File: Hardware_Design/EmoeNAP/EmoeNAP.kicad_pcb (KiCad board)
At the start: 4 copper layers, 75 x 36 mm, 149 parts, among them J1 Power, J2 10Hz to WIDEBAND, J3 10Hz to 1MHz, J4 Input, J5 10Hz to 100kHz, U1 OPA1612, U2 OPA1612, U3 OPA1612, U4 PS-12E05, U5 OPA1612, U6 OPA1679, U7 OPA1612, U8 OPA1612

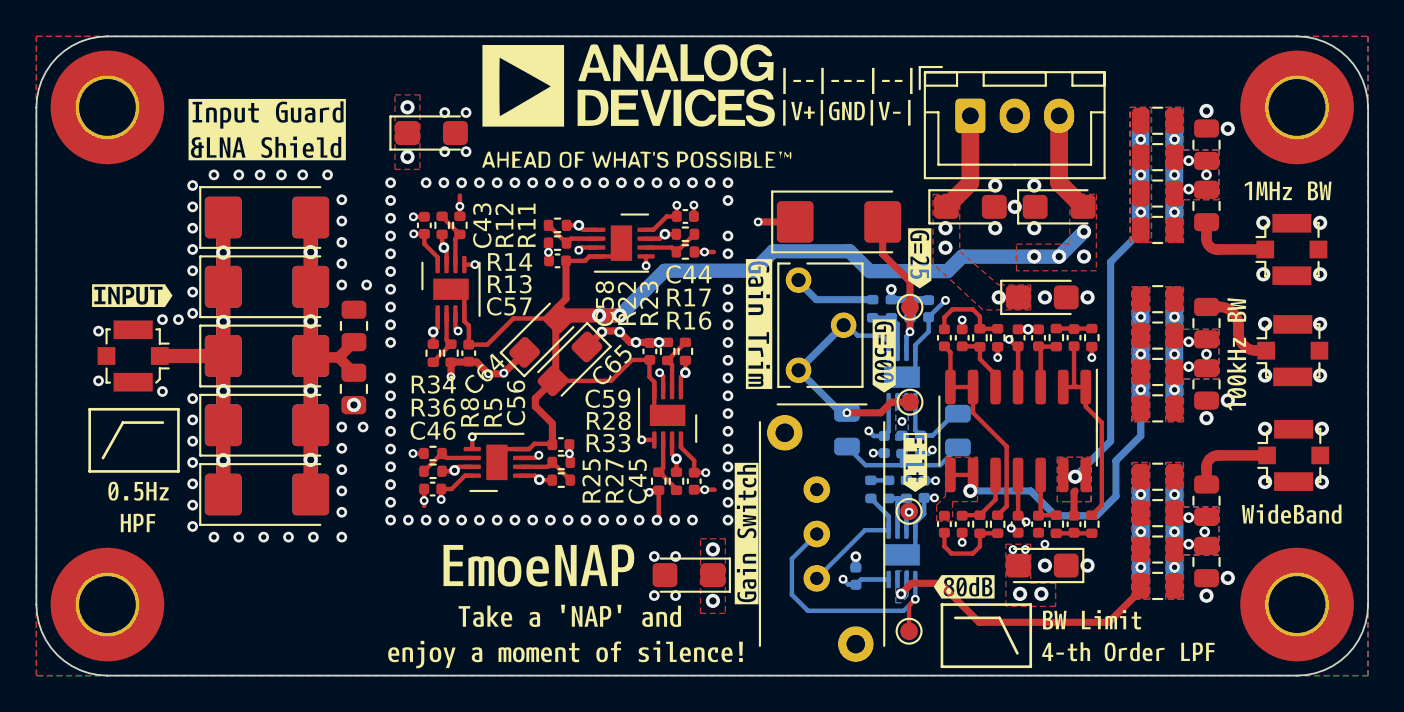
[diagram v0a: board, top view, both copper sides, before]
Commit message: Update EmoeNAP design
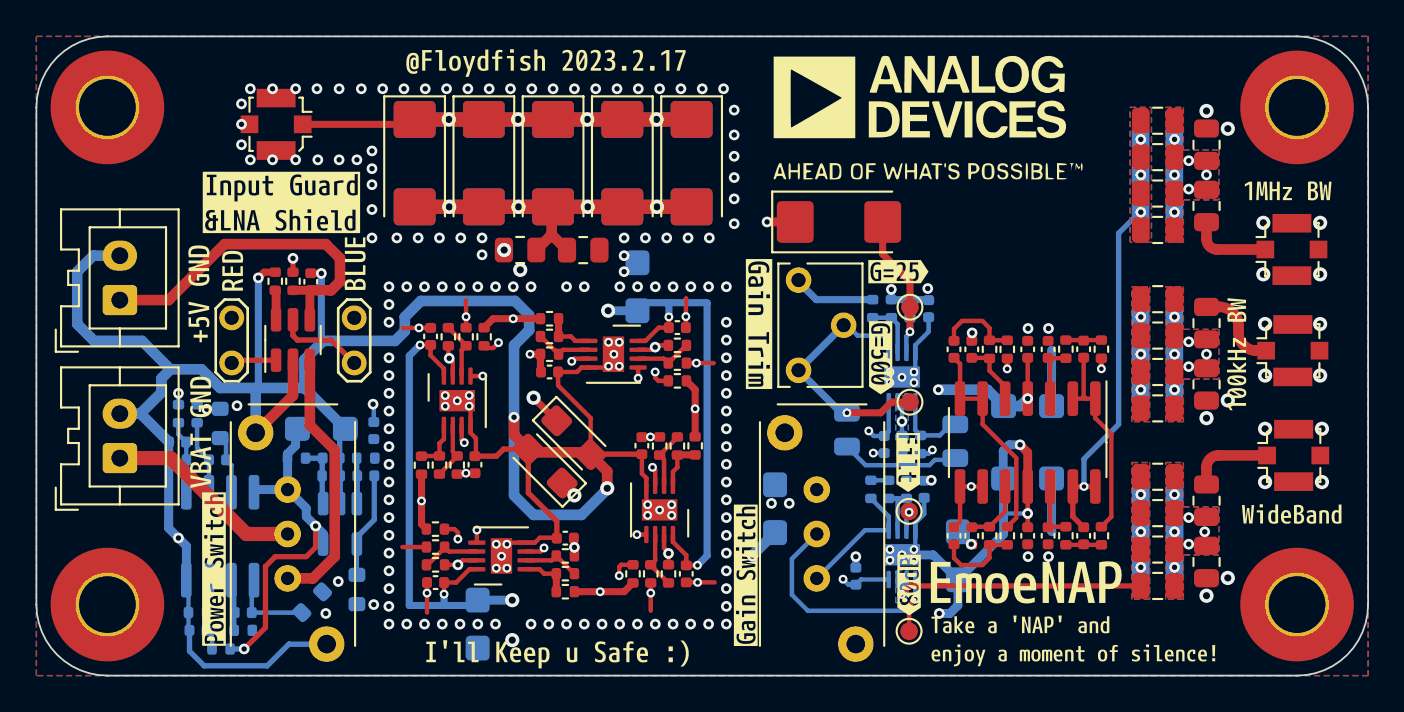
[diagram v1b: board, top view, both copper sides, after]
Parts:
- removed kibuzzard-6378A5E8: G***, kibuzzard-6378A5E8
- removed kibuzzard-6378A61B: G***, kibuzzard-6378A61B
- removed kibuzzard-6378A7B0: G***, kibuzzard-6378A7B0
- removed kibuzzard-6378A846: G***, kibuzzard-6378A846
- removed kibuzzard-6378A8BF: G***, kibuzzard-6378A8BF
- removed kibuzzard-6378AB08: G***, kibuzzard-6378AB08
- added C65: 2.2uF, Capacitor_Tantalum_SMD:CP_EIA-3216-10_Kemet-I, B.Cu at (126.0, 111.1)
- added C66: 100pF, Capacitor_SMD:C_0402_1005Metric, B.Cu at (119.1, 122.5)
- added C67: 100pF, Capacitor_SMD:C_0402_1005Metric, B.Cu at (121.7, 121.5)
- added C68: 100pF, Capacitor_SMD:C_0402_1005Metric, B.Cu at (118.0, 111.8)
- added C69: 100pF, Capacitor_SMD:C_0402_1005Metric, B.Cu at (120.2, 112.8)
- added C70: 0.1uF, Capacitor_SMD:C_0402_1005Metric, B.Cu at (129.0, 111.2)
- added C71: 0.1uF, Capacitor_SMD:C_0402_1005Metric, F.Cu at (125.5, 102.8)
- added C72: 100pF, Capacitor_SMD:C_0402_1005Metric, B.Cu at (126.6, 112.8)
- added C73: 100pF, Capacitor_SMD:C_0402_1005Metric, B.Cu at (128.6, 113.8)
- added J6: GREEN, TestPoint:TestPoint_2Pads_Pitch2.54mm_Drill0.8mm, F.Cu at (127.9, 104.9)
- added J7: RED, TestPoint:TestPoint_2Pads_Pitch2.54mm_Drill0.8mm, F.Cu at (121.0, 104.8)
- added J8: USB_CHR, Connector_JST:JST_XA_B02B-XASK-1_1x02_P2.50mm_Vertical, F.Cu at (114.7, 103.8)
- added R12: 1R, Resistor_SMD:R_0402_1005Metric, F.Cu at (146.1, 108.4)
- added R15: 1R, Resistor_SMD:R_0402_1005Metric, F.Cu at (147.1, 112.1)
- added R18: 1R, Resistor_SMD:R_0402_1005Metric, F.Cu at (143.6, 119.3)
- added R24: 1R, Resistor_SMD:R_0402_1005Metric, F.Cu at (139.8, 120.3)
- added R3: 1R, Resistor_SMD:R_0402_1005Metric, F.Cu at (138.9, 104.9)
- added R30: 1R, Resistor_SMD:R_0402_1005Metric, F.Cu at (132.5, 116.7)
- added R34: 1R, Resistor_SMD:R_0402_1005Metric, F.Cu at (131.7, 113.1)
- added R41: 1R, Resistor_SMD:R_0402_1005Metric, F.Cu at (135.2, 105.9)
- added R45: 10k, Resistor_SMD:R_0402_1005Metric, B.Cu at (120.4, 123.5)
- added R46: 10k, Resistor_SMD:R_0402_1005Metric, B.Cu at (119.1, 121.5)
- added R47: 1k, Resistor_SMD:R_0402_1005Metric, B.Cu at (121.7, 122.5)
- added R48: 10k, Resistor_SMD:R_0402_1005Metric, B.Cu at (118.0, 110.2)
- added R49: 10k, Resistor_SMD:R_0402_1005Metric, B.Cu at (117.9, 112.8)
- added R50: 1k, Resistor_SMD:R_0402_1005Metric, B.Cu at (119.0, 110.2)
- added R51: 2k, Resistor_SMD:R_0402_1005Metric, F.Cu at (123.5, 102.8)
- added R52: 1k, Resistor_SMD:R_0402_1005Metric, F.Cu at (124.5, 102.8)
- added R53: 10k, Resistor_SMD:R_0402_1005Metric, B.Cu at (124.7, 112.8)
- added R54: 10k, Resistor_SMD:R_0402_1005Metric, B.Cu at (126.6, 113.8)
- added R55: 1k, Resistor_SMD:R_0402_1005Metric, B.Cu at (128.6, 112.8)
- added RISO5: 100R, Resistor_SMD:R_0603_1608Metric, B.Cu at (125.5, 120.9)
- added RISO6: 100R, Resistor_SMD:R_0603_1608Metric, B.Cu at (120.3, 110.8)
- added RISO7: 100R, Resistor_SMD:R_0603_1608Metric, B.Cu at (128.1, 120.2)
- added U10: PS-12E05, EmoeNAP_FootPrint_Lib:PS-12E05, F.Cu at (124.2, 114.5)
- added U11: TP4057, Package_TO_SOT_SMD:SOT-23-6, F.Cu at (124.5, 106.1)
- added U12: SGM321, Package_TO_SOT_SMD:SOT-23-5, B.Cu at (127.1, 116.5)
- added U9: LT1364, Package_SO:SOIC-8_3.9x4.9mm_P1.27mm, B.Cu at (120.3, 117.2)
- added kibuzzard-63ED0A5F: G***, kibuzzard-63ED0A5F, F.Cu at (168.4, 123.0)
- added kibuzzard-63EE512D: G***, kibuzzard-63EE512D, F.Cu at (120.0, 119.0)
- added kibuzzard-63EE51C1: G***, kibuzzard-63EE51C1, F.Cu at (119.2, 103.5)
- added kibuzzard-63EE51DC: G***, kibuzzard-63EE51DC, F.Cu at (119.2, 111.3)
- added kibuzzard-63EE520C: G***, kibuzzard-63EE520C, F.Cu at (121.0, 102.2)
- added kibuzzard-63EE5216: G***, kibuzzard-63EE5216, F.Cu at (128.0, 101.8)
- added kibuzzard-63EE5345: G***, kibuzzard-63EE5345, F.Cu at (138.7, 90.5)
- added kibuzzard-63EE53DB: G***, kibuzzard-63EE53DB, F.Cu at (139.3, 123.8)
- C50: renamed from C51; moved to B.Cu
- C51: renamed from C52; moved to B.Cu
- C52: renamed from C53; moved to B.Cu
- C53: renamed from C54; moved to B.Cu
- C63: renamed from C66; moved to B.Cu
- C64: renamed from C67; moved to B.Cu
- G***: moved to B.Cu
- J1: value Power -> Battery; footprint Connector_JST:JST_XH_B3B-XH-A_1x03_P2.50mm_Vertical -> Connector_JST:JST_XA_B02B-XASK-1_1x02_P2.50mm_Vertical
- moved J1 51.6 mm to (114.7, 112.8), turned to 90 degrees
- moved G*** 51.3 mm to (165.6, 101.0)
- moved G*** 36.5 mm to (155.2, 95.8), turned to 180 degrees
- moved kibuzzard-6378A590 27.5 mm to (165.8, 119.8)
- moved C20 24.1 mm to (146.9, 96.1), turned to -90 degrees
- moved C23 24.1 mm to (146.9, 96.1), turned to -90 degrees
- moved C18 21.2 mm to (143.0, 96.1), turned to -90 degrees
- moved C26 21.2 mm to (143.0, 96.1), turned to -90 degrees
- moved C64 20.5 mm to (161.9, 118.2), turned to -90 degrees
- moved C11 20.4 mm to (131.3, 96.1), turned to -90 degrees
- moved C31 20.4 mm to (131.3, 96.1), turned to -90 degrees
- moved C53 20.2 mm to (151.6, 115.6), turned to 90 degrees
- moved C44 20.1 mm to (146.6, 119.3), turned to -90 degrees
- moved C15 19.4 mm to (139.1, 96.1), turned to -90 degrees
- moved C28 19.4 mm to (139.1, 96.1), turned to -90 degrees
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- renumbered C56 to C54, C57 to C55, C58 to C56, C59 to C57, C60 to C58, C61 to C59, C62 to C60, C64 to C61, C65 to C62, R9 to R10, R10 to R11, R11 to R13, R12 to R14, R13 to R16, R14 to R17, R15 to R19, R16 to R20, R17 to R21, R18 to R22, R19 to R23, R20 to R25, R21 to R26, R22 to R27, R23 to R28, R24 to R29, R25 to R31, R26 to R32, R27 to R33, R28 to R35, R29 to R36, R30 to R37, R31 to R38, R32 to R39, R3 to R4, R33 to R40, R34 to R42, R35 to R43, R36 to R44, R4 to R5, R5 to R6, R6 to R7, R7 to R8, R8 to R9, TP4 to TP3, TP3 to TP4
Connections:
- J1 pad 1: VDD -> /VBAT
- J1 pad 2: GND -> VSS
- R14 pad 1: Net-(C1-Pad1) -> Net-(R12-Pad1)
- R17 pad 1: Net-(C1-Pad1) -> Net-(R15-Pad1)
- R21 pad 1: Net-(C1-Pad1) -> Net-(R18-Pad1)
- R28 pad 1: Net-(C1-Pad1) -> Net-(R24-Pad1)
- R33 pad 1: Net-(C1-Pad1) -> Net-(R30-Pad1)
- R40 pad 1: Net-(C1-Pad1) -> Net-(R34-Pad1)
- R44 pad 1: Net-(C1-Pad1) -> Net-(R41-Pad1)
- R9 pad 1: Net-(C1-Pad1) -> Net-(R3-Pad1)
- U1 pad 1: Net-(C1-Pad1) -> Net-(R3-Pad1)
- U1 pad 7: Net-(C1-Pad1) -> Net-(R12-Pad1)
- U5 pad 1: Net-(C1-Pad1) -> Net-(R15-Pad1)
- U5 pad 7: Net-(C1-Pad1) -> Net-(R18-Pad1)
- U7 pad 1: Net-(C1-Pad1) -> Net-(R24-Pad1)
- U7 pad 7: Net-(C1-Pad1) -> Net-(R30-Pad1)
- U8 pad 1: Net-(C1-Pad1) -> Net-(R34-Pad1)
- U8 pad 7: Net-(C1-Pad1) -> Net-(R41-Pad1)
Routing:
- net VSS: track 132.3 -> 232.3 mm, vias 13 -> 38
- net VDD: track 145.0 -> 212.1 mm, vias 14 -> 17
- net /VBUS_+5V: track 0.00 -> 19.9 mm
- net /VBAT_CHRG: track 0.00 -> 14.8 mm
- net Net-(C1-Pad1): track 68.1 -> 82.2 mm, vias 9 -> 5
- net Net-(J6-Pad1): track 0.00 -> 12.7 mm, vias 0 -> 1
- net /VBAT: track 0.00 -> 11.2 mm
- net Net-(R18-Pad1): track 0.00 -> 6.79 mm, vias 0 -> 2
- net Net-(R41-Pad1): track 0.00 -> 6.53 mm, vias 0 -> 2
- net Net-(C73-Pad2): track 0.00 -> 5.59 mm
- net Net-(J6-Pad2): track 0.00 -> 4.98 mm
- net Net-(RISO3-Pad2): track 74.0 -> 69.5 mm
- net Net-(R30-Pad1): track 0.00 -> 4.57 mm, vias 0 -> 2
- net Net-(C67-Pad2): track 0.00 -> 4.52 mm
- net Net-(R12-Pad1): track 0.00 -> 4.34 mm, vias 0 -> 2
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- added copper zone on B.Cu, net Net-(R6-Pad1)
- removed copper zone on B.Cu, net Net-(R7-Pad1)
- removed copper zone on F.Cu, net VDD
- removed copper zone on In2.Cu, net VDD
- removed copper zone on F.Cu, net VSS
